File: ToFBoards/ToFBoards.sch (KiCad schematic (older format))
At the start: 1 part, among them U1 VL53L1X

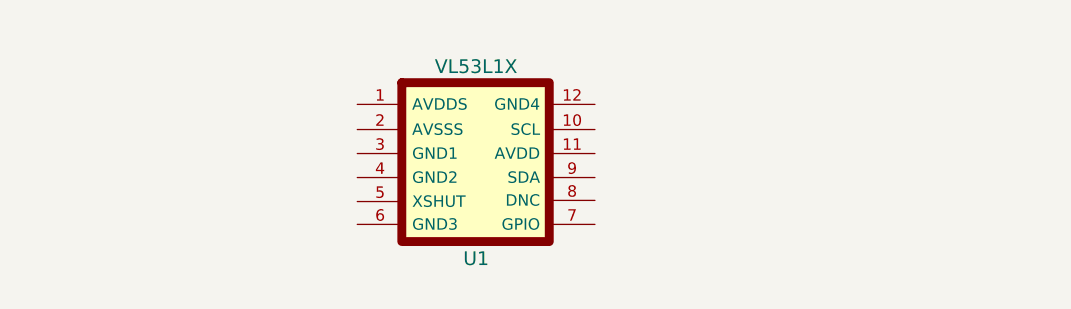
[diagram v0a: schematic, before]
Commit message: ToF boards
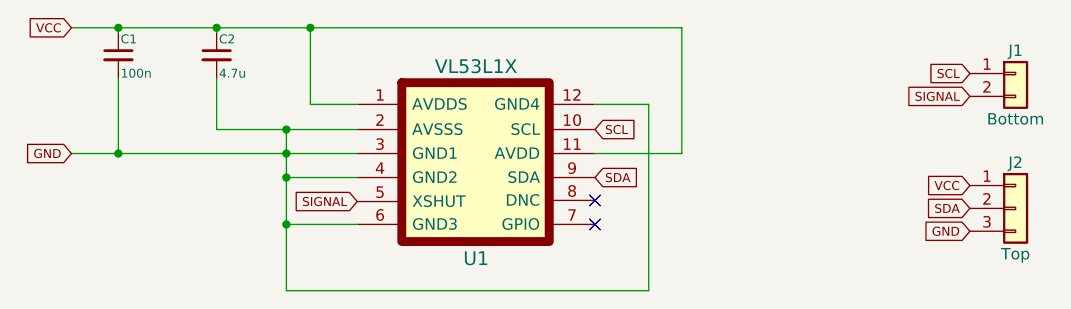
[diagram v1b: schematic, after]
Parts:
- added C1: 100n, Capacitors_SMD:C_0402, symbol C_Small
- added C2: 4.7u, Capacitors_SMD:C_0402, symbol C_Small
- added J1: Bottom, footprint:ToFTop, symbol Conn_01x02
- added J2: Top, footprint:ToFBottom, symbol Conn_01x03
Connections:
- net VCC: now reaches U1.1 (AVDDS)
- net VCC: now also U1.11 (AVDD), C1.1, C2.1, J2.1 (Pin_1)
- net SCL: now reaches U1.10 (SCL)
- net SCL: now also J1.1 (Pin_1)
- net GND: now reaches U1.12 (GND4)
- net GND: now also U1.2 (AVSSS), U1.3 (GND1), U1.4 (GND2), U1.6 (GND3), C1.2, C2.2, J2.3 (Pin_3)
- net SIGNAL: now reaches U1.5 (XSHUT)
- net SIGNAL: now also J1.2 (Pin_2)
- net SDA: now reaches U1.9 (SDA)
- net SDA: now also J2.2 (Pin_2)
- no-connect marks 0 -> 2
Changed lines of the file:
@@
 LIBS:valves
 LIBS:parts
+LIBS:ToFBoards-cache
 EELAYER 25 0
 EELAYER END
@@
 	1    0    0    -1
 $EndComp
+Text GLabel 6185 3545 2    39   Input ~ 0
+SCL
+Text GLabel 6185 3755 2    39   Input ~ 0
+SDA
+$Comp
+L C_Small C2
+U 1 1 5B60667F
+P 4530 3220
+F 0 "C2" H 4540 3290 39  0000 L CNN
+F 1 "4.7u" H 4540 3140 39  0000 L CNN
+F 2 "Capacitors_SMD:C_0402" H 4530 3220 50  0001 C CNN
+F 3 "" H 4530 3220 50  0001 C CNN
+	1    4530 3220
+	1    0    0    -1
+$EndComp
+$Comp
+L C_Small C1
+U 1 1 5B606704
+P 4100 3220
+F 0 "C1" H 4110 3290 39  0000 L CNN
+F 1 "100n" H 4110 3140 39  0000 L CNN
+F 2 "Capacitors_SMD:C_0402" H 4100 3220 50  0001 C CNN
+F 3 "" H 4100 3220 50  0001 C CNN
+	1    4100 3220
+	1    0    0    -1
+$EndComp
+Text GLabel 3895 3100 0    39   Input ~ 0
+VCC
+Text GLabel 3895 3650 0    39   Input ~ 0
+GND
+Text GLabel 5145 3860 0    39   Input ~ 0
+SIGNAL
+NoConn ~ 6185 3855
+NoConn ~ 6185 3960
+Wire Wire Line
+	5145 3960 4835 3960
+Wire Wire Line
+	4835 3545 4835 4250
+Wire Wire Line
+	4835 3755 5145 3755
+Wire Wire Line
+	6185 3435 6420 3435
+Wire Wire Line
+	6420 3435 6420 4250
+Wire Wire Line
+	6420 4250 4835 4250
+Connection ~ 4835 3960
+Wire Wire Line
+	3895 3100 6565 3100
+Wire Wire Line
+	4100 3100 4100 3120
+Wire Wire Line
+	4530 3100 4530 3120
+Connection ~ 4100 3100
+Wire Wire Line
+	6565 3100 6565 3650
+Wire Wire Line
+	6565 3650 6185 3650
+Connection ~ 4530 3100
+Wire Wire Line
+	5145 3435 4940 3435
+Wire Wire Line
+	4940 3435 4940 3100
+Connection ~ 4940 3100
+Wire Wire Line
+	4100 3320 4100 3650
+Wire Wire Line
+	3895 3650 5145 3650
+Connection ~ 4100 3650
+Connection ~ 4835 3650
+Connection ~ 4835 3755
+Wire Wire Line
+	4530 3545 5145 3545
+Wire Wire Line
+	4530 3320 4530 3545
+Connection ~ 4835 3545
+$Comp
+L Conn_01x02 J1
+U 1 1 5B606E26
+P 8025 3300
+F 0 "J1" H 8025 3400 50  0000 C CNN
+F 1 "Bottom" H 8025 3100 50  0000 C CNN
+F 2 "footprint:ToFTop" H 8025 3300 50  0001 C CNN
+F 3 "" H 8025 3300 50  0001 C CNN
+	1    8025 3300
+	1    0    0    -1
+$EndComp
+$Comp
+L Conn_01x03 J2
+U 1 1 5B606EF1
+P 8025 3890
+F 0 "J2" H 8025 4090 50  0000 C CNN
+F 1 "Top" H 8025 3690 50  0000 C CNN
+F 2 "footprint:ToFBottom" H 8025 3890 50  0001 C CNN
+F 3 "" H 8025 3890 50  0001 C CNN
+	1    8025 3890
+	1    0    0    -1
+$EndComp
+Text GLabel 7825 3890 0    39   Input ~ 0
+SDA
+Text GLabel 7825 3790 0    39   Input ~ 0
+VCC
+Text GLabel 7825 3990 0    39   Input ~ 0
+GND
+Text GLabel 7825 3400 0    39   Input ~ 0
+SIGNAL
+Text GLabel 7825 3300 0    39   Input ~ 0
+SCL
 $EndSCHEMATC
